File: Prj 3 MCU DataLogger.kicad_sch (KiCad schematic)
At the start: 25 parts, among them U1 24LC1025, U2 24LC1025, U3 DS1337S_, U4 ATMEGA328P-AU, Y1 16 MHz, Y2 32.768 KHz

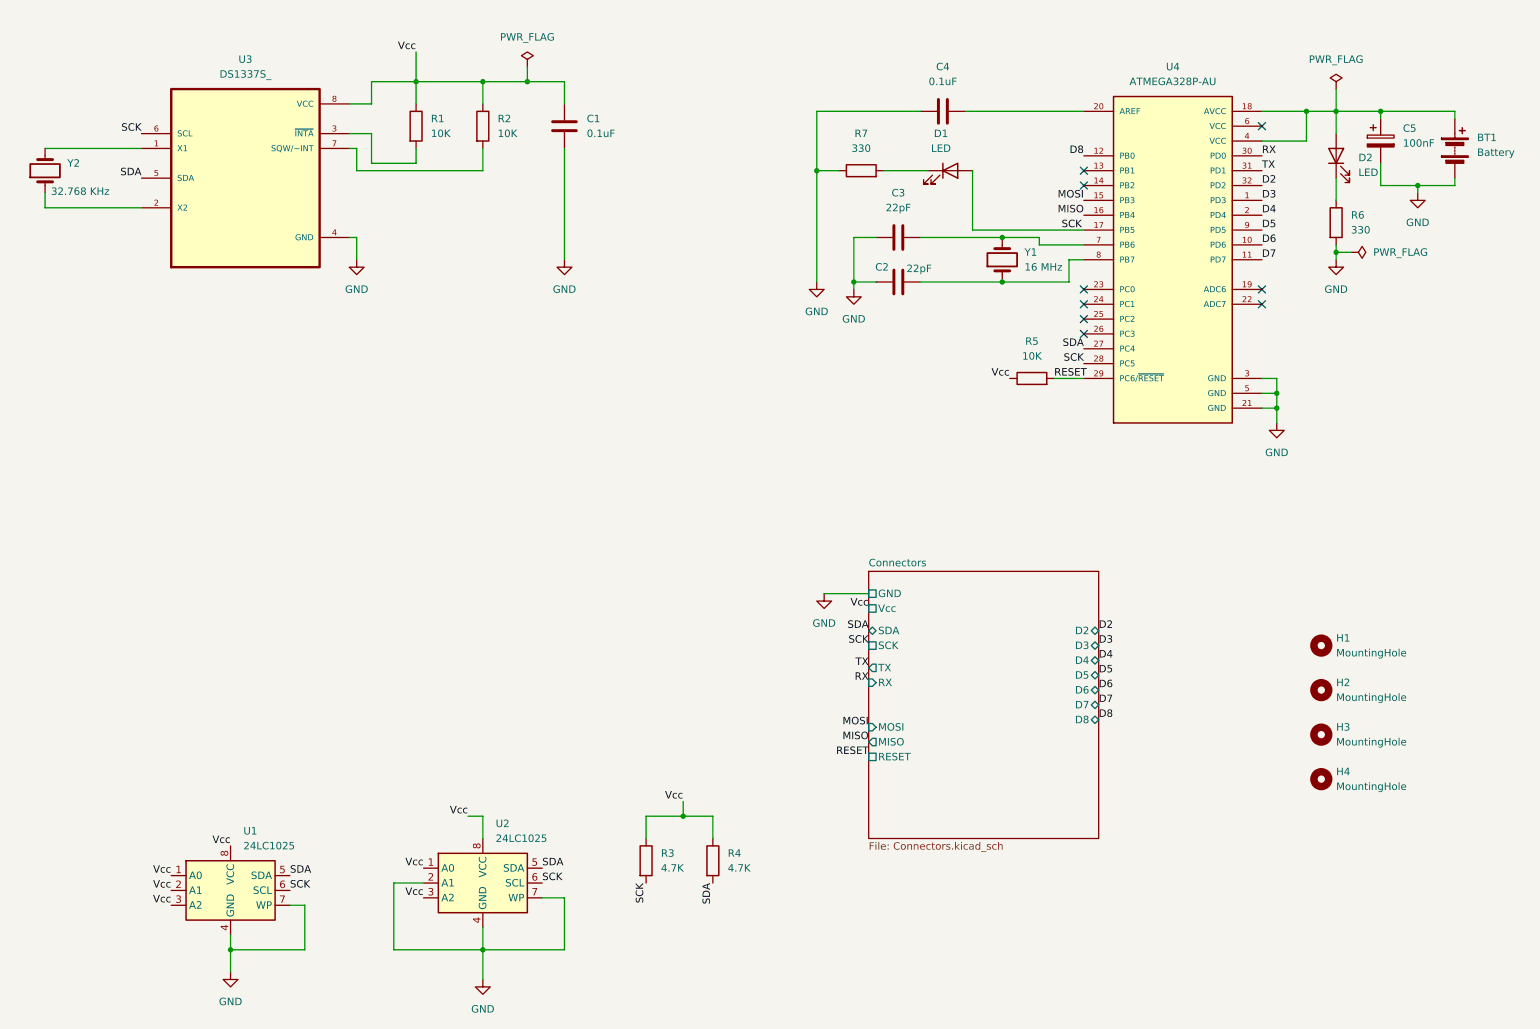
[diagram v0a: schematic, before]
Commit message: Comments completed.
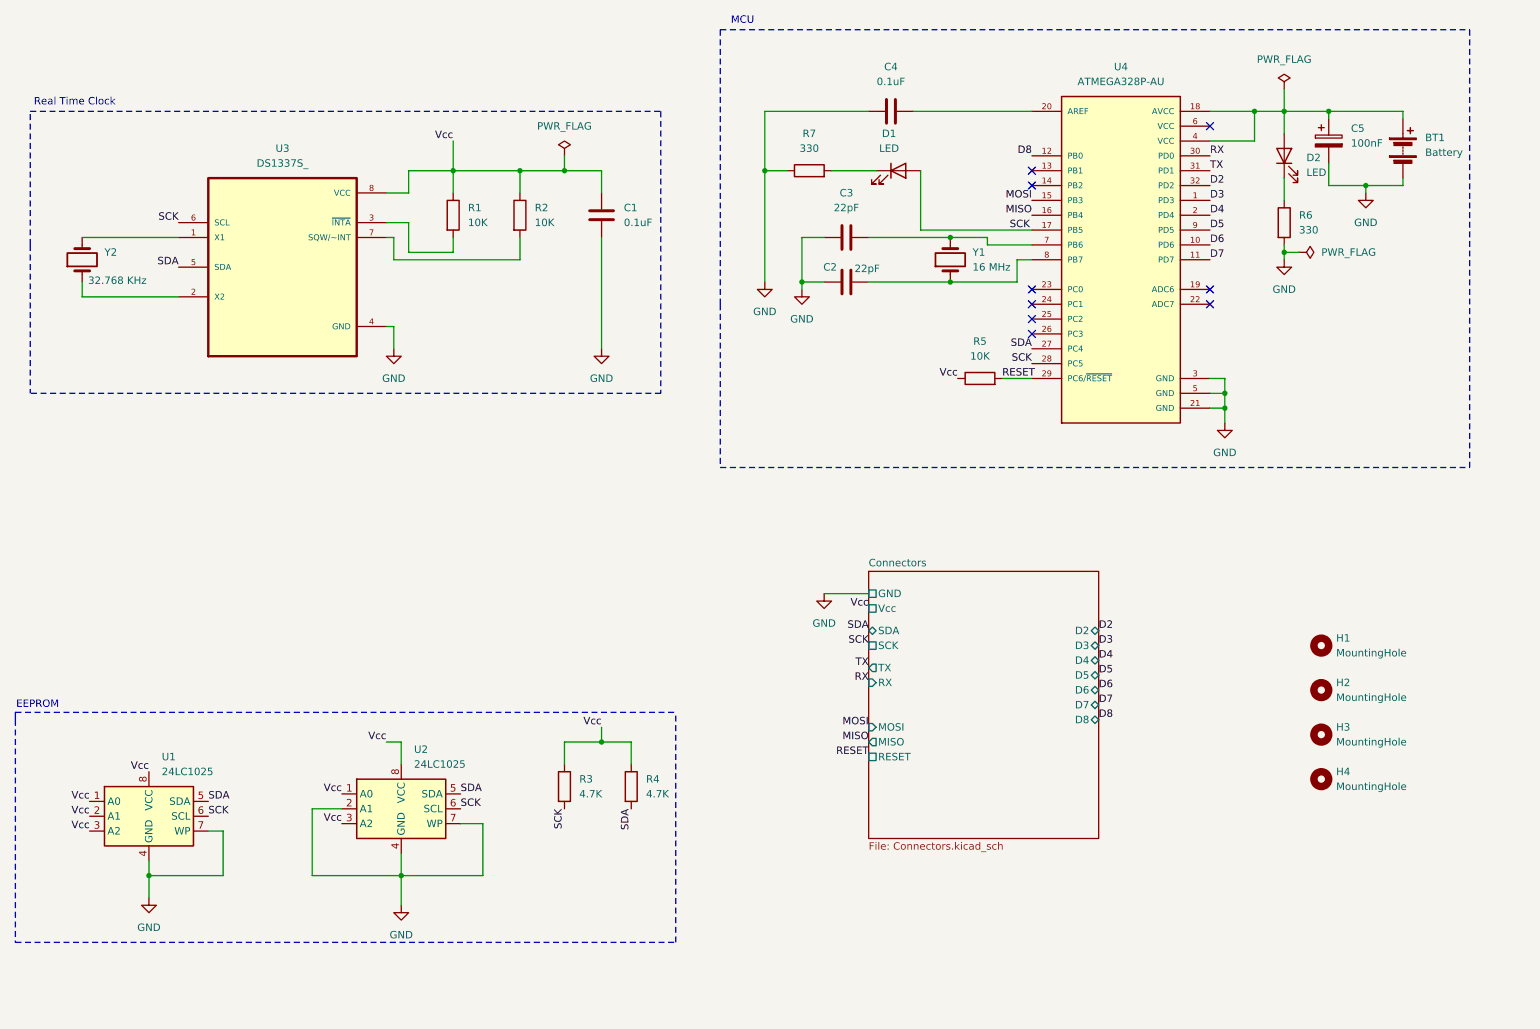
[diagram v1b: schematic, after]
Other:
- note added: "EEPROM"
- note added: "MCU"
- note added: "Real Time Clock"
- moved on the sheet: BT1, C1, C2, C3, C4, C5, D1, D2, R1, R2, R3, R4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
